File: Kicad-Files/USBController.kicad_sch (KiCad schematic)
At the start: 16 parts, among them IC1 TUSB7320, Y1 48 MHz

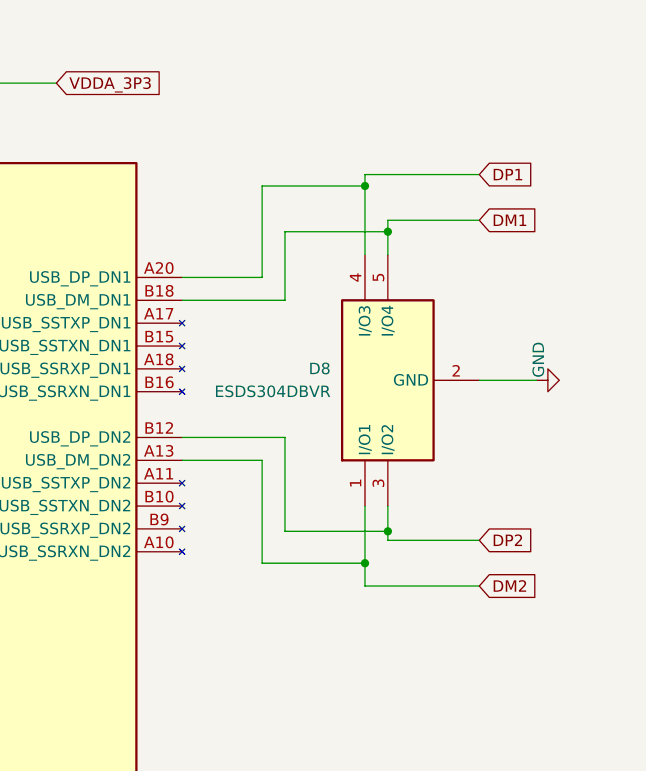
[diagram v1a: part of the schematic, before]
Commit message: fixed pdf schematics, removed temporary files
Signed-off-by: Jakub Sobota <jakub.sobota@3mdeb.com>
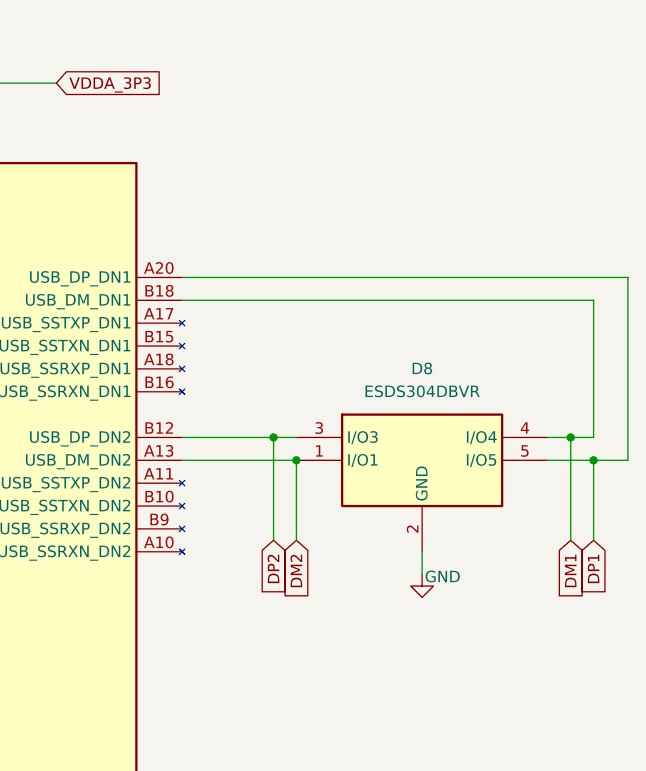
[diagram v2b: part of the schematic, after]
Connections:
- net DM1: now also D8.4 (I/O4); no longer D8.5 (I/O4)
- net DP1: now also D8.5 (I/O5); no longer D8.4 (I/O3)
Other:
- moved on the sheet: D8
